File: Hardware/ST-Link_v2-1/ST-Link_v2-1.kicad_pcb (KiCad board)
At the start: 2 copper layers, 26.3 x 17.7 mm, 42 parts, among them J1 Conn_01x06, J2 USB_C_Receptacle, U1 STM32F103CBTx, U2 LP5907MFX-3.3, Y1 8Mhz

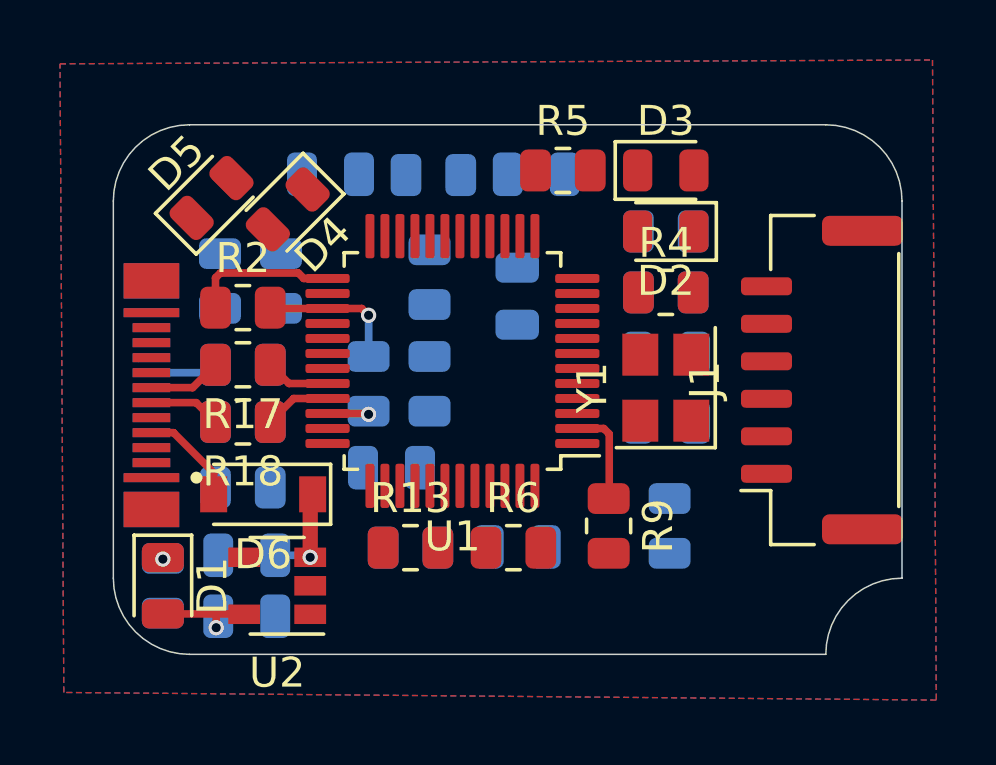
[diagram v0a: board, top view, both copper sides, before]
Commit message: 5/12/2021
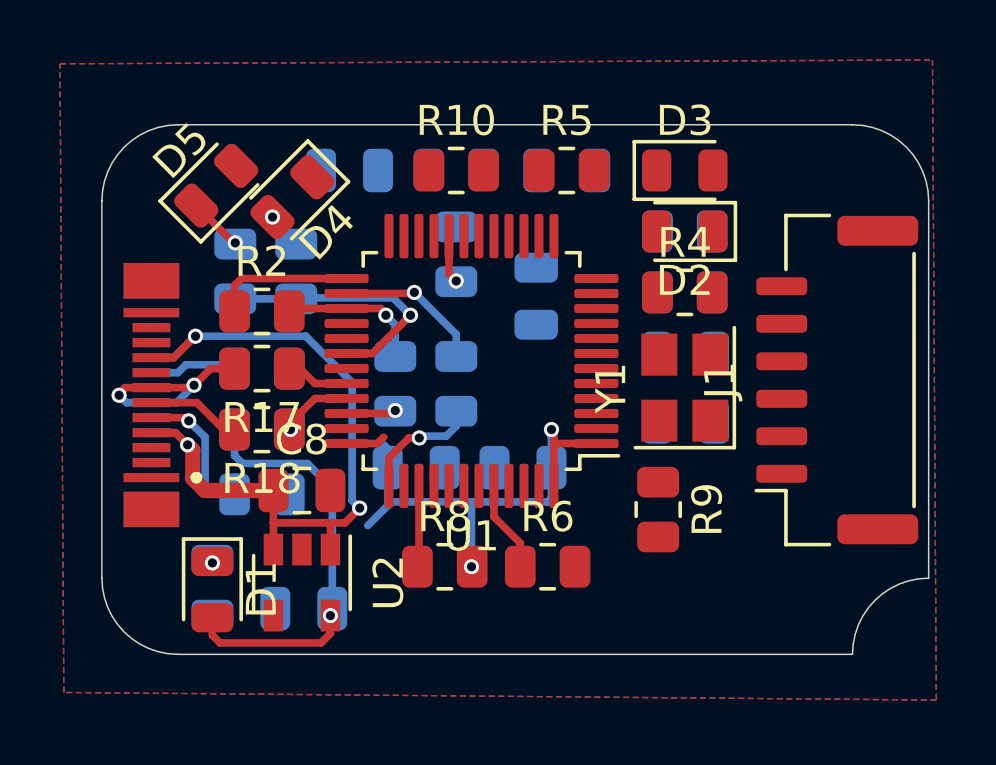
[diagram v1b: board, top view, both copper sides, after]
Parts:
- removed D6: 1N4001, HKUST_RT_BJT:D_SOD-123
- removed R13: 100R, HKUST_RT_RCL:R_0805_2012Metric
- C8, R10, R8: moved to F.Cu
- R14, R15: value 4.7k -> 10k
- moved R10 13.8 mm to (189.1, 129.8), turned to 0 degrees
- moved C8 2.84 mm to (184.0, 140.5), turned to 0 degrees
- moved C7 2.65 mm to (191.3, 139.7)
- moved C9 1.92 mm to (184.0, 144.4), turned to 180 degrees
- moved R9 1.74 mm to (195.8, 141.1)
- moved D1 1.66 mm to (181.0, 143.8)
- moved R3 1.65 mm to (181.0, 143.7)
- moved R6 1.31 mm to (192.2, 143.0)
- moved R8 1.31 mm to (188.7, 143.0)
- moved R7 1.17 mm to (189.1, 132.6), turned to 90 degrees
- moved C1 1.02 mm to (192.8, 129.8)
- moved R19 0.89 mm to (189.1, 136.9)
- moved R20 0.89 mm to (187.1, 136.9)
- moved U2 0.83 mm to (184.0, 143.5), turned to 270 degrees
- moved C6 0.83 mm to (187.8, 139.7)
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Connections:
- net /SWCLK renamed /JTCK
- net /SWDIO renamed /JTMS
- net /SWDIO_IN renamed Net-(R2-Pad1)
- J2 pad A4: Net-(D6-Pad2) -> +5V
- J2 pad A9: Net-(D6-Pad2) -> +5V
- J2 pad B4: Net-(D6-Pad2) -> +5V
- J2 pad B9: Net-(D6-Pad2) -> +5V
- U1 pad 21: Net-(U1-Pad21) -> Net-(R10-Pad1)
- U1 pad 3: Net-(R10-Pad1) -> Net-(U1-Pad3)
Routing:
- net +3V3: track 3.23 -> 31.8 mm, vias 1 -> 3
- net +5V: track 3.33 -> 27.6 mm, vias 1 -> 3
- net /LED_STLINK: track 0.00 -> 8.75 mm, vias 0 -> 1
- net /JTCK: track 0.00 -> 4.98 mm, vias 0 -> 1
- net Net-(J2-PadA5): track 0.00 -> 4.80 mm, vias 0 -> 1
- net Net-(J2-PadA7): track 2.58 -> 7.09 mm, vias 0 -> 2
- net /ST_SWCLK: track 0.00 -> 4.11 mm, vias 0 -> 1
- net Net-(D6-Pad2): track 3.78 -> 0.00 mm
- net Net-(R9-Pad1): track 3.63 -> 0.00 mm
- net Net-(R6-Pad1): track 0.00 -> 3.06 mm
- net Net-(R8-Pad1): track 0.00 -> 2.78 mm
- net Net-(R7-Pad1): track 0.00 -> 1.60 mm, vias 0 -> 1
- net Net-(J2-PadB5): track 2.19 -> 3.07 mm
- net Net-(J2-PadA6): track 2.40 -> 3.14 mm
- net Net-(D5-Pad1): track 0.48 -> 1.13 mm, vias 0 -> 1
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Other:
- board size 26.3 x 17.7 mm -> 27.6 x 17.7 mm

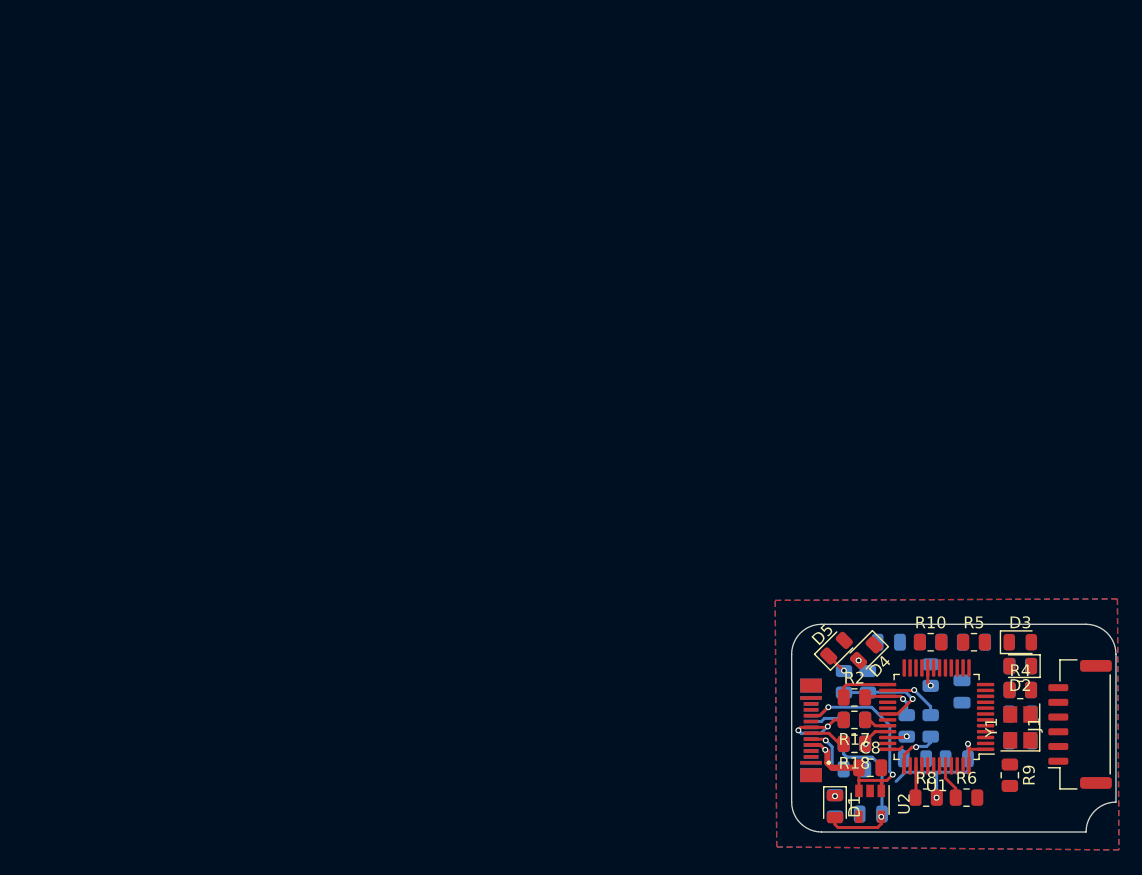
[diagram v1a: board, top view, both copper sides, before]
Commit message: V2.1 11/12/2021
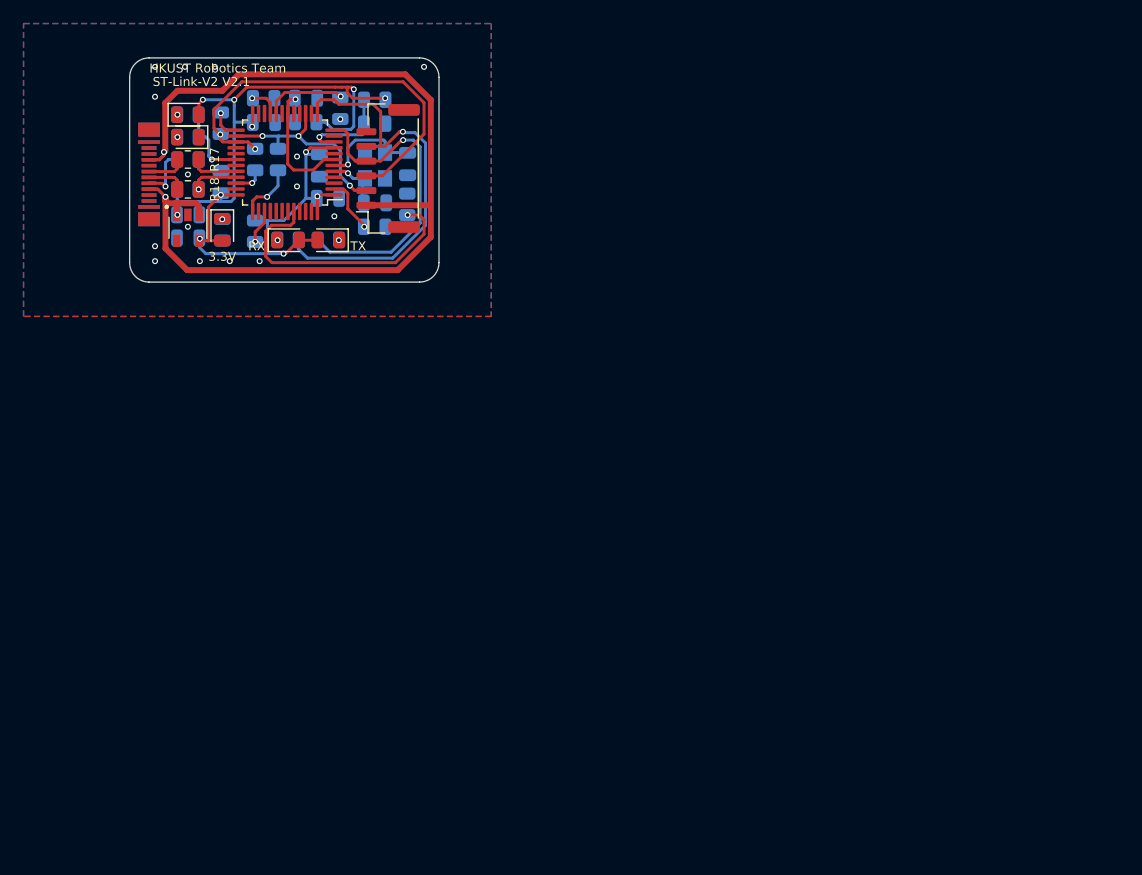
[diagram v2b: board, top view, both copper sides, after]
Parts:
- removed J2: USB_C_Receptacle, HKUST_RT_CONN:USB_C_MALE
- removed R21: 5.1k, HKUST_RT_RCL:R_0805_2012Metric
- added P1: USB_C_Plug_USB2.0, HKUST_RT_CONN:USB_C_MALE, F.Cu at (122.7, 90.0)
- C8, R10, R2, R4, R5, R6, R8, R9, Y1: moved to B.Cu
- moved C6 77.4 mm to (132.4, 85.6)
- moved C4 76.4 mm to (128.8, 90.7)
- moved C9 75.9 mm to (126.0, 95.4)
- moved U2 75.9 mm to (126.0, 94.6)
- moved J1 75.4 mm to (143.0, 89.5)
- moved R8 74.6 mm to (131.7, 94.9), turned to 90 degrees
- moved C8 74.6 mm to (126.0, 93.5)
- moved R14 74.3 mm to (141.9, 83.7)
- moved R12 74.0 mm to (126.0, 86.9), turned to 180 degrees
- moved R17 74.0 mm to (126.0, 88.8)
- moved R22 74.0 mm to (126.0, 88.8)
- moved C7 74.0 mm to (137.2, 89.3), turned to 270 degrees
- moved R11 73.7 mm to (126.0, 85.0), turned to 0 degrees
- moved R16 73.7 mm to (126.0, 91.3)
- moved R18 73.7 mm to (126.0, 91.3)
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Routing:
- net +5V: track 27.6 -> 86.4 mm
- net +3V3: track 31.8 -> 82.1 mm, vias 3 -> 10
- net /RXD: track 0.00 -> 35.9 mm, vias 0 -> 1
- net /JTMS: track 4.89 -> 34.8 mm, vias 1 -> 2
- net /TXD: track 0.00 -> 27.0 mm, vias 0 -> 1
- net Net-(R6-Pad1): track 3.06 -> 23.2 mm, vias 0 -> 1
- net /NRST: track 0.00 -> 12.6 mm, vias 0 -> 1
- net /JTCK: track 4.98 -> 17.4 mm, vias 1 -> 3
- net Net-(C3-Pad1): track 0.00 -> 9.03 mm, vias 0 -> 1
- net Net-(R14-Pad1): track 0.00 -> 8.31 mm, vias 0 -> 1
- net Net-(R7-Pad1): track 1.60 -> 7.30 mm
- net Net-(J2-PadA5): track 4.80 -> 0.00 mm, vias 1 -> 0
- net Net-(R9-Pad1): track 0.00 -> 4.75 mm, vias 0 -> 1
- net Net-(C2-Pad1): track 0.00 -> 4.37 mm, vias 0 -> 1
- net Net-(P1-PadA7): track 7.09 -> 3.27 mm, vias 2 -> 0
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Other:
- board size 27.6 x 17.7 mm -> 26.3 x 19 mm
- board text added: "11/12/2021"
- board text added: "3.3V"
- board text added: "HKUST Robotics Team"
- board text added: "RX"
- board text added: "ST-Link-V2 V2.1"
- board text added: "TX"
- board text added: "by Samson"
